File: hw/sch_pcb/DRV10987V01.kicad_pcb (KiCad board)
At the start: 2 copper layers, 50.3 x 40.1 mm, 30 parts, among them IC1 DRV10987DPWPR, J10 PWR, J11 WAGO, J12 WAGO, J2 I2C, J3 HEADER_2x04_PARALLEL, J5 AUX, J6 MOTOR, M1 HOLE M3, M2 HOLE M3, M3 HOLE M3, M4 HOLE M3

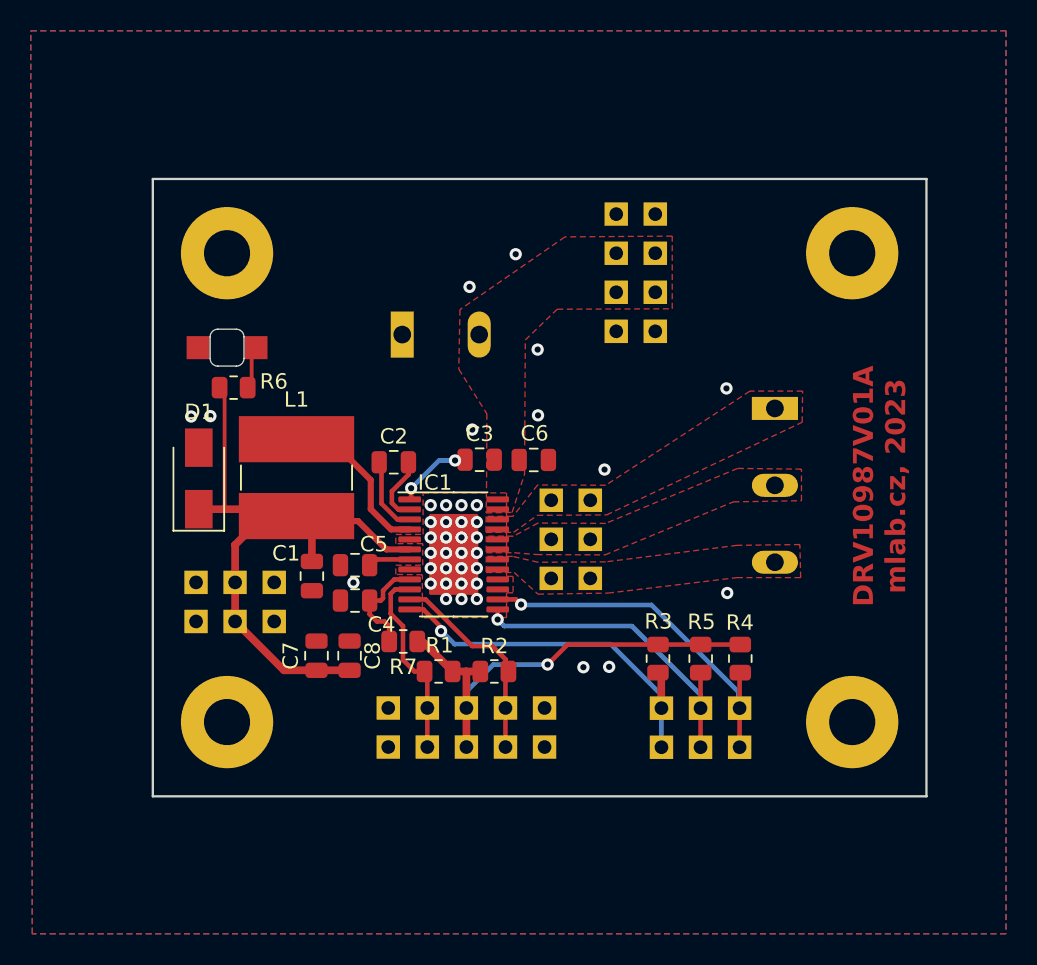
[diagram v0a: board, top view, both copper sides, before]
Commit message: Edit PCB and schema
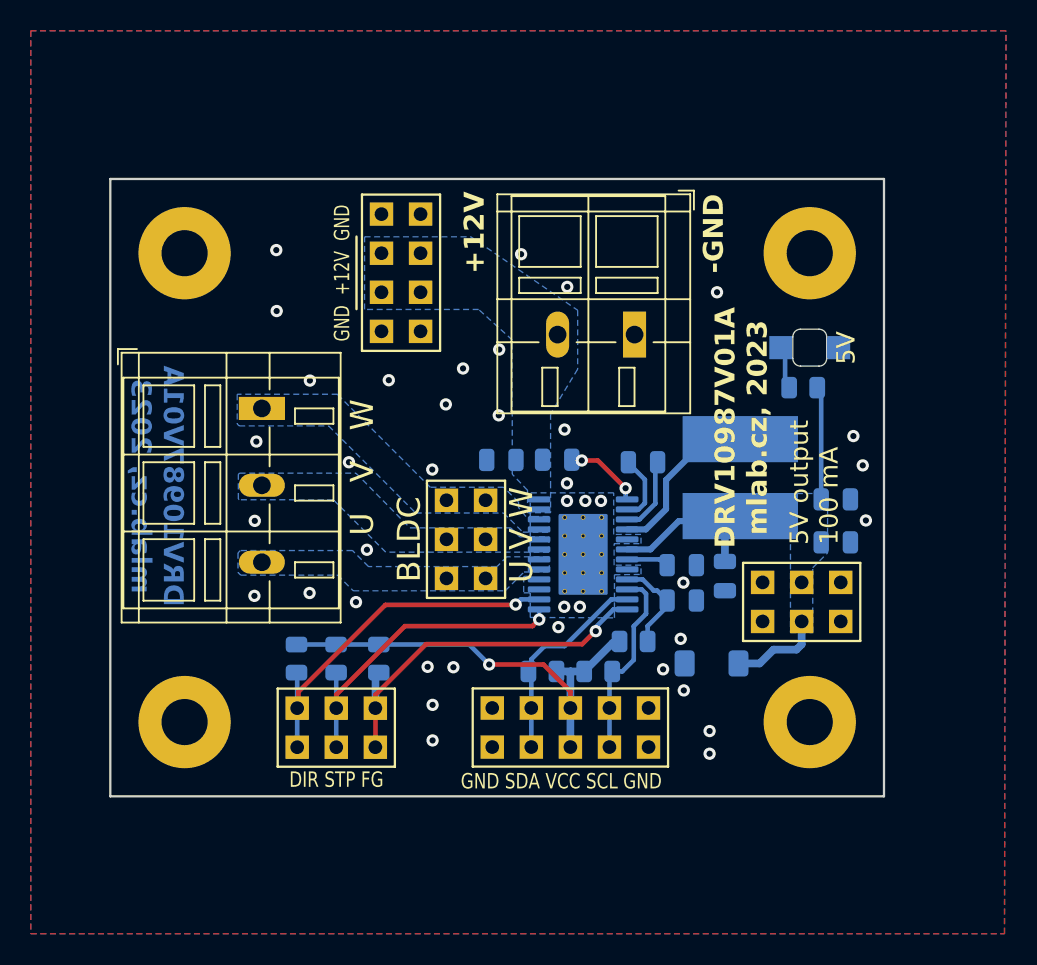
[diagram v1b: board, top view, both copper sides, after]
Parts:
- C1, C3, C4, C5, C6, C7, C8, D2, IC1, L1, R1, R2, R3, R4, R5, R6, R7: moved to B.Cu
- C2: value 100nF -> 10nF; moved to B.Cu
- D1: footprint Diode_SMD:D_SMA -> Diode_SMD:D_MiniMELF; moved to B.Cu
- J10, J11, J12, J2, J3, J5, J6, M1, M2, M3, M4: moved to F.Cu
- moved M2 43.4 mm to (125.4, 89.8), turned to 0 degrees
- moved M4 43.4 mm to (125.4, 120.2), turned to 0 degrees
- moved D2 37.9 mm to (166.1, 95.9), turned to 0 degrees
- moved M1 37.9 mm to (166.1, 89.8), turned to 0 degrees
- moved M3 37.9 mm to (166.1, 120.2), turned to 0 degrees
- moved R6 37.0 mm to (165.6, 98.5), turned to 0 degrees
- moved J10 36.8 mm to (165.5, 112.4)
- moved D1 35.4 mm to (159.7, 116.4), turned to 180 degrees
- moved C7 34.6 mm to (167.8, 108.6), turned to 0 degrees
- moved J12 33.3 mm to (130.4, 99.8)
- moved C8 33.2 mm to (167.8, 105.8), turned to 0 degrees
- moved L1 28.8 mm to (161.5, 104.3)
- moved R4 28.8 mm to (132.7, 116.1)
- moved C1 26.8 mm to (160.5, 110.8)
- moved R5 23.7 mm to (135.3, 116.1)
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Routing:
- net +5V: track 39.6 -> 22.7 mm
- net /V3P3: track 6.93 -> 6.34 mm
- added copper zone on B.Cu, net +12V
- added copper zone on B.Cu, net +5V
- added copper zone on B.Cu, net /U
- added copper zone on B.Cu, net /V
- added copper zone on B.Cu, net /W
- removed copper zone on F.Cu, net +12V
- removed copper zone on F.Cu, net /U
- removed copper zone on F.Cu, net /V
- removed copper zone on F.Cu, net /W
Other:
- rule pad_to_mask_clearance: 0 -> 0.2
- board text added: "W V U"
- board text removed: "U V W"
